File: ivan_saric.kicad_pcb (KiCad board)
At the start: 2 copper layers, 62.7 x 90 mm, 0 parts

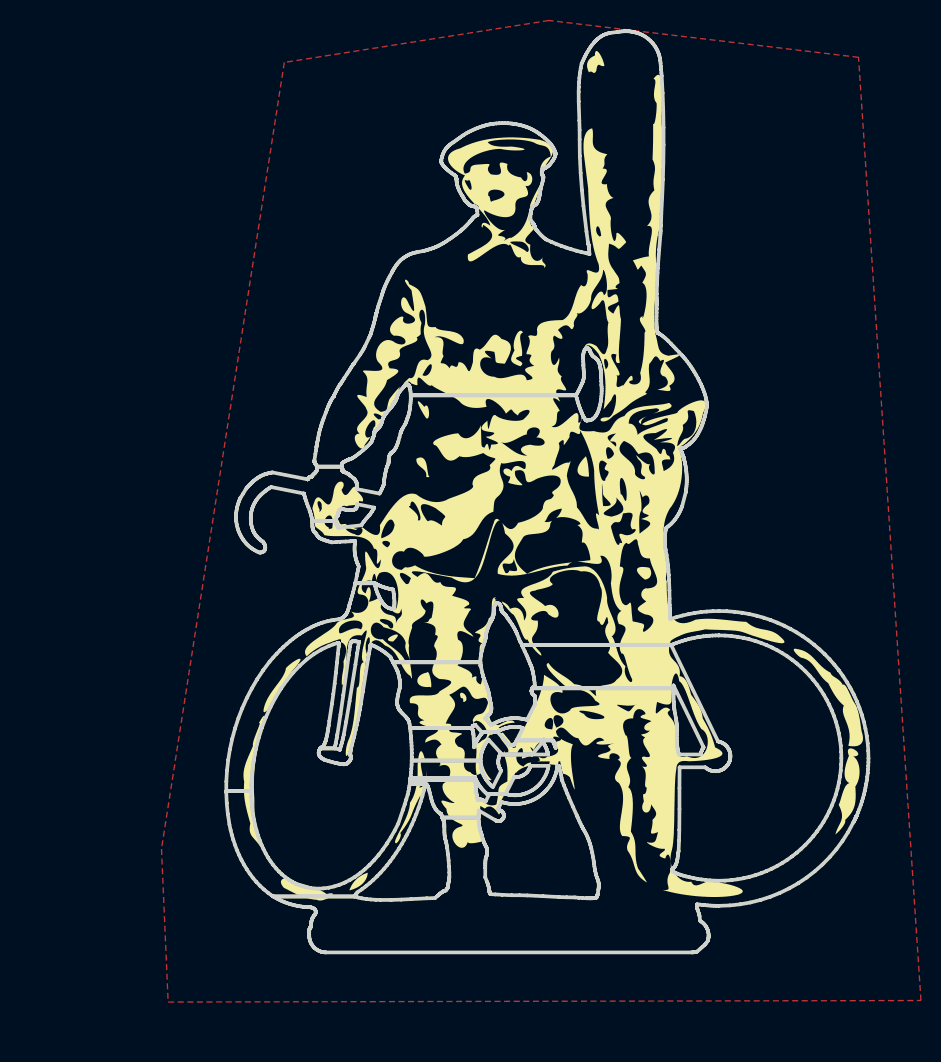
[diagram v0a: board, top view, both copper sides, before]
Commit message: plated version
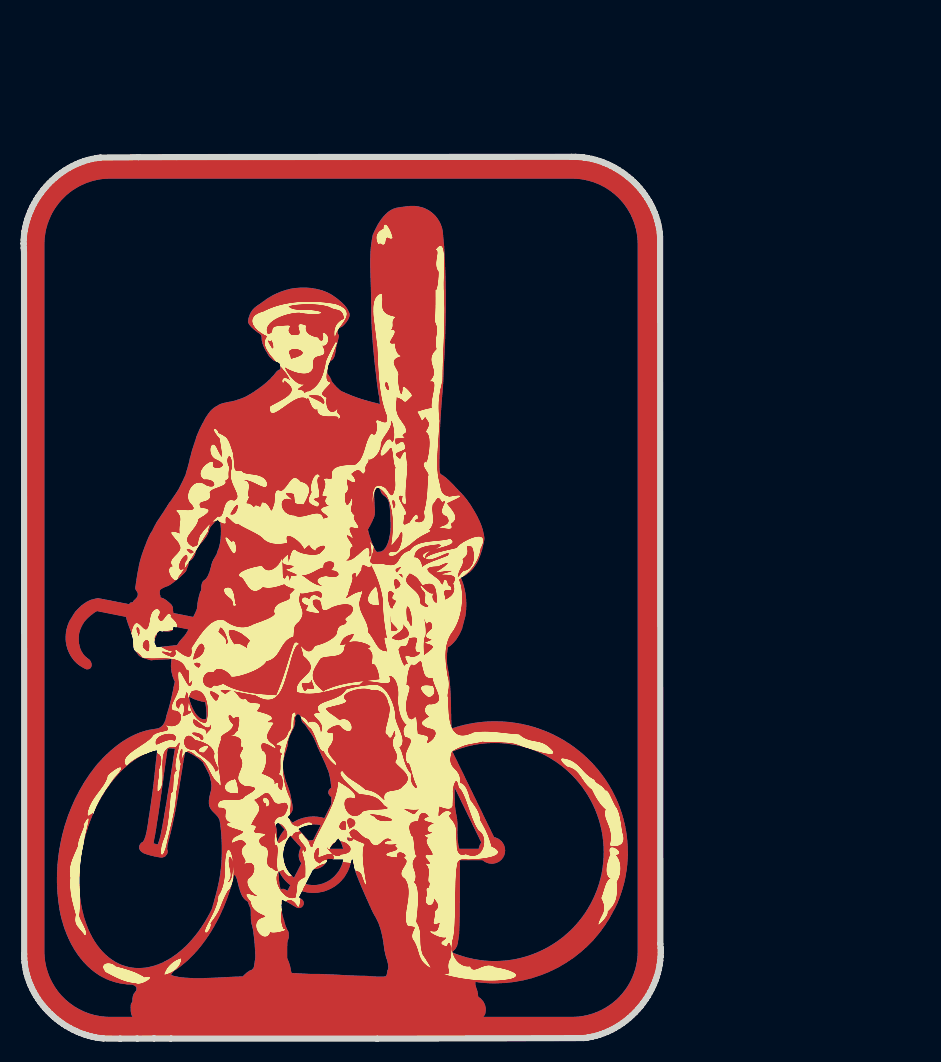
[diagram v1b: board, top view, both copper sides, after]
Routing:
- removed copper zone on F.Cu, net (none)
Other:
- board size 62.7 x 90 mm -> 62.3 x 86.2 mm
